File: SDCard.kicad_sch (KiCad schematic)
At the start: 4 parts, among them J4 Micro_SD_Card_Det

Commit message: workday
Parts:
- R12, R13: footprint Resistor_SMD:R_0603_1608Metric -> Resistor_SMD:R_0603_1608Metric_Pad0.98x0.95mm_HandSolder
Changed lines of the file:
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@@
 			)
 		)
-		(property "Footprint" "Resistor_SMD:R_0603_1608Metric"
+		(property "Footprint" "Resistor_SMD:R_0603_1608Metric_Pad0.98x0.95mm_HandSolder"
 			(at 168.91 105.283 90)
 			(effects
@@
 			)
 		)
-		(property "Footprint" "Resistor_SMD:R_0603_1608Metric"
+		(property "Footprint" "Resistor_SMD:R_0603_1608Metric_Pad0.98x0.95mm_HandSolder"
 			(at 165.862 114.935 90)
 			(effects

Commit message: tweaking
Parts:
- J4: footprint SD_CARD:microSD_HC_Hirose_DM3AT-SF-PEJM5 -> Connector_Card:microSD_HC_Hirose_DM3AT-SF-PEJM5
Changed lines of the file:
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@@
 			)
 		)
-		(property "Footprint" "SD_CARD:microSD_HC_Hirose_DM3AT-SF-PEJM5"
+		(property "Footprint" "Connector_Card:microSD_HC_Hirose_DM3AT-SF-PEJM5"
 			(at 253.365 80.645 0)
 			(effects

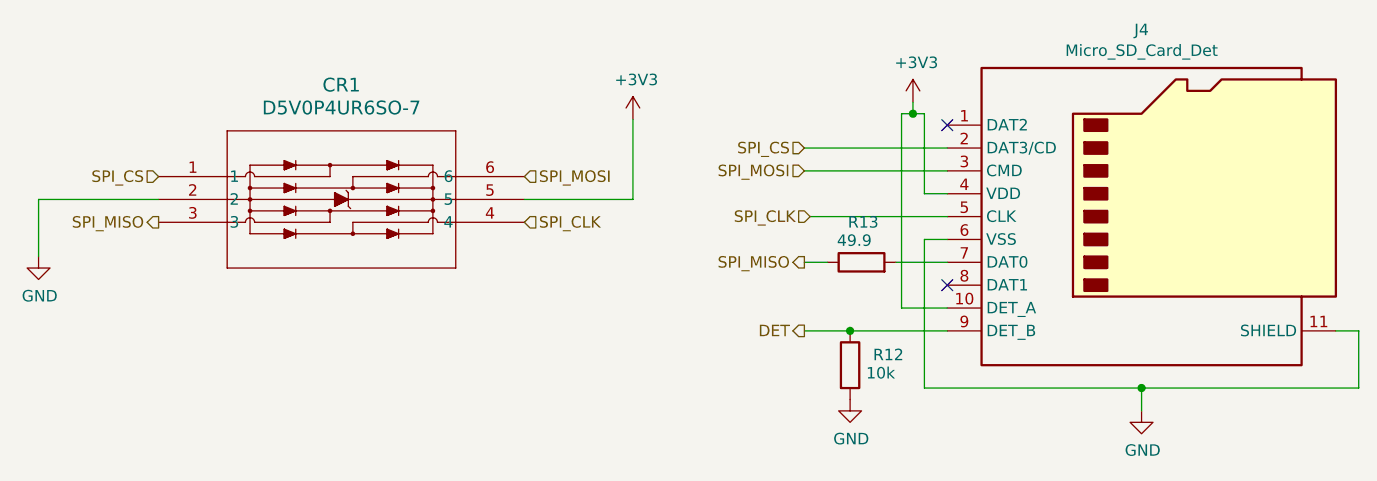
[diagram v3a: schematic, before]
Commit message: bom
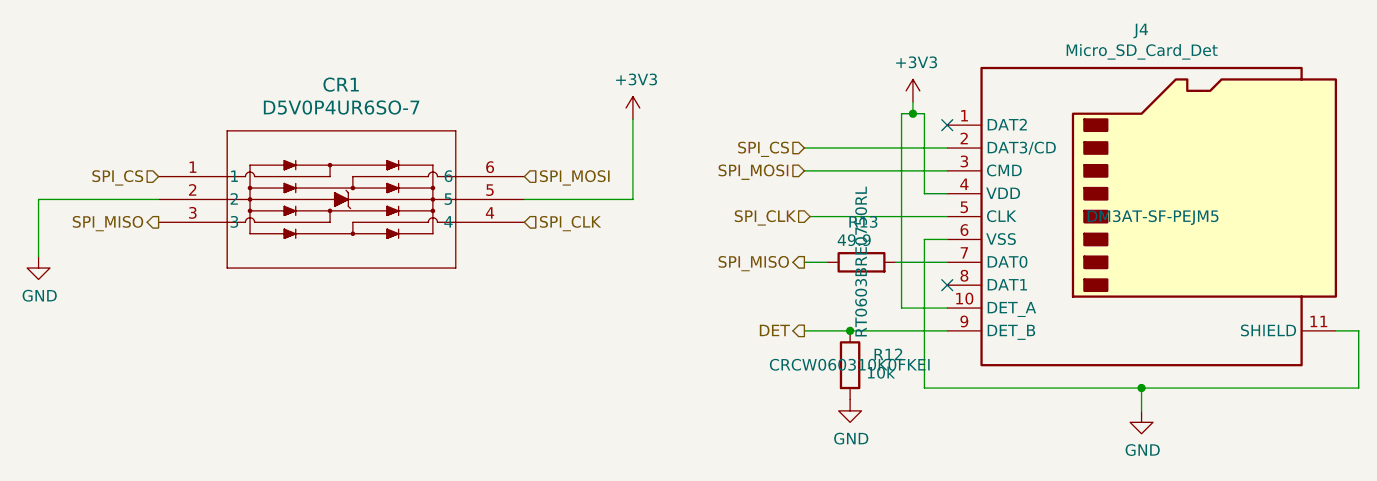
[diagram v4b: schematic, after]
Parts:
- J4: Mouser Part Number (none) -> DM3AT-SF-PEJM5
- R12: Mouser Part Number (none) -> CRCW060310K0FKEI
- R13: Mouser Part Number (none) -> RT0603BRE0750RL
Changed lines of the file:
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@@
+			)
+		)
+		(property "Mouser Part Number" "RT0603BRE0750RL"
+			(at 168.91 103.505 0)
+			(effects
+				(font
+					(size 1.27 1.27)
+				)
 			)
 		)
@@
 			)
 		)
+		(property "Mouser Part Number" "DM3AT-SF-PEJM5"
+			(at 201.295 98.425 0)
+			(effects
+				(font
+					(size 1.27 1.27)
+				)
+			)
+		)
 		(pin "1"
 		)
@@
 			(at 167.64 114.935 0)
 			(effects
+				(font
+					(size 1.27 1.27)
+				)
+			)
+		)
+		(property "Mouser Part Number" "CRCW060310K0FKEI "
+			(at 167.64 114.935 0)
+			(effects

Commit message: updated pins
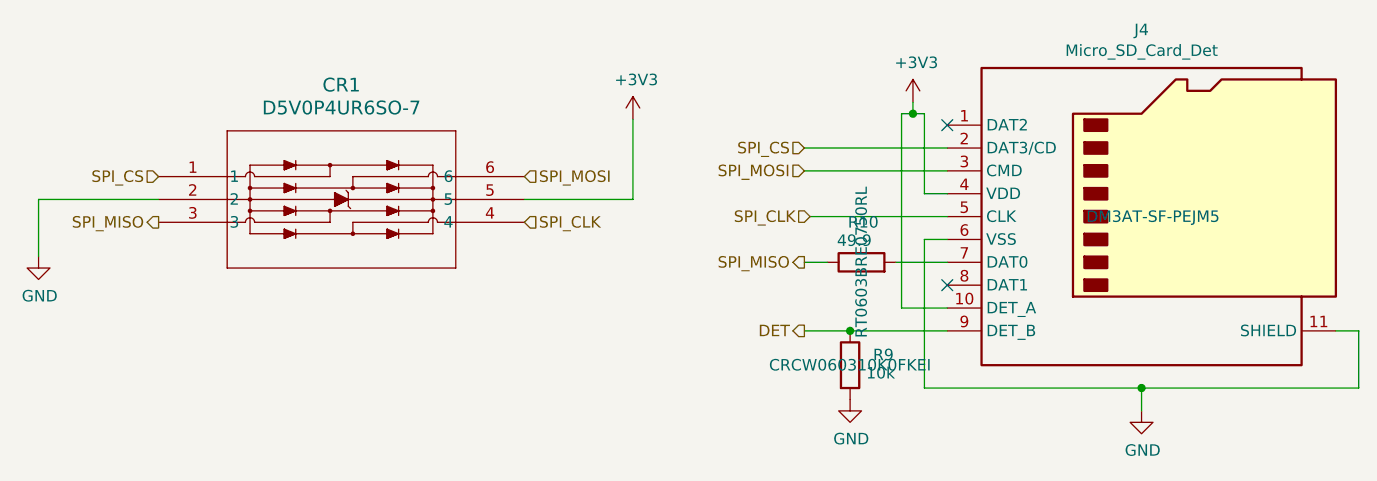
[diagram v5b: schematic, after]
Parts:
- renumbered R13 to R10, R12 to R9
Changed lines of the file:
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@@
 		(on_board yes)
 		(dnp no)
-		(property "Reference" "#PWR038"
+		(property "Reference" "#PWR030"
 			(at 167.64 125.095 0)
 			(effects
@@
 			(project "LeaderSOM"
 				(path "/192d0c36-944e-4927-949b-263b8c85a7ca/54eecd34-7b2b-4895-a003-33708e7ad7e6"
-					(reference "#PWR038")
+					(reference "#PWR030")
 					(unit 1)
 				)
@@
 		(on_board yes)
 		(dnp no)
-		(property "Reference" "#PWR039"
+		(property "Reference" "#PWR031"
 			(at 174.625 89.535 0)
 			(effects
@@
 			(project "LeaderSOM"
 				(path "/192d0c36-944e-4927-949b-263b8c85a7ca/54eecd34-7b2b-4895-a003-33708e7ad7e6"
-					(reference "#PWR039")
+					(reference "#PWR031")
 					(unit 1)
 				)
@@
 		(on_board yes)
 		(dnp no)
-		(property "Reference" "R13"
+		(property "Reference" "R10"
 			(at 170.815 99.06 90)
 			(effects
@@
 			(project "LeaderSOM"
 				(path "/192d0c36-944e-4927-949b-263b8c85a7ca/54eecd34-7b2b-4895-a003-33708e7ad7e6"
-					(reference "R13")
+					(reference "R10")
 					(unit 1)
 				)
@@
 		(on_board yes)
 		(dnp no)
-		(property "Reference" "#PWR040"
+		(property "Reference" "#PWR032"
 			(at 200.025 126.365 0)
 			(effects
@@
 			(project "LeaderSOM"
 				(path "/192d0c36-944e-4927-949b-263b8c85a7ca/54eecd34-7b2b-4895-a003-33708e7ad7e6"
-					(reference "#PWR040")
+					(reference "#PWR032")
 					(unit 1)
 				)
@@
 		(on_board yes)
 		(dnp no)
-		(property "Reference" "#PWR036"
+		(property "Reference" "#PWR028"
 			(at 77.47 109.22 0)
 			(effects
@@
 			(project "LeaderSOM"
 				(path "/192d0c36-944e-4927-949b-263b8c85a7ca/54eecd34-7b2b-4895-a003-33708e7ad7e6"
-					(reference "#PWR036")
+					(reference "#PWR028")
 					(unit 1)
 				)
@@
 		(on_board yes)
 		(dnp no)
-		(property "Reference" "#PWR037"
+		(property "Reference" "#PWR029"
 			(at 143.51 91.44 0)
 			(effects
@@
 			(project "LeaderSOM"
 				(path "/192d0c36-944e-4927-949b-263b8c85a7ca/54eecd34-7b2b-4895-a003-33708e7ad7e6"
-					(reference "#PWR037")
+					(reference "#PWR029")
 					(unit 1)
 				)
@@
 		(on_board yes)
 		(dnp no)
-		(property "Reference" "R12"
+		(property "Reference" "R9"
 			(at 170.18 113.792 0)
 			(effects
@@
 			(project "LeaderSOM"
 				(path "/192d0c36-944e-4927-949b-263b8c85a7ca/54eecd34-7b2b-4895-a003-33708e7ad7e6"
-					(reference "R12")
-					(unit 1)
-				)
+					(reference "R9")
+					(unit 1)
+				)
